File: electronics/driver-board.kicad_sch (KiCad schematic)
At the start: 62 parts, among them J10 USB_C_Receptacle_USB2.0, J2 Conn_01x02, J3 Conn_01x06, J4 Qwiic_RA, J5 Conn_02x03_Counter_Clockwise, SW1 SW_Push, SW2 SW_Push, SW3 SW_Push, SW4 SW_Push, U1 LMR16006YQ3, U2 AMS1117-3.3, U3 ESP32-C6-MINI-1/U, U5 TMC5240-TSSOP38, U7 AS5047D

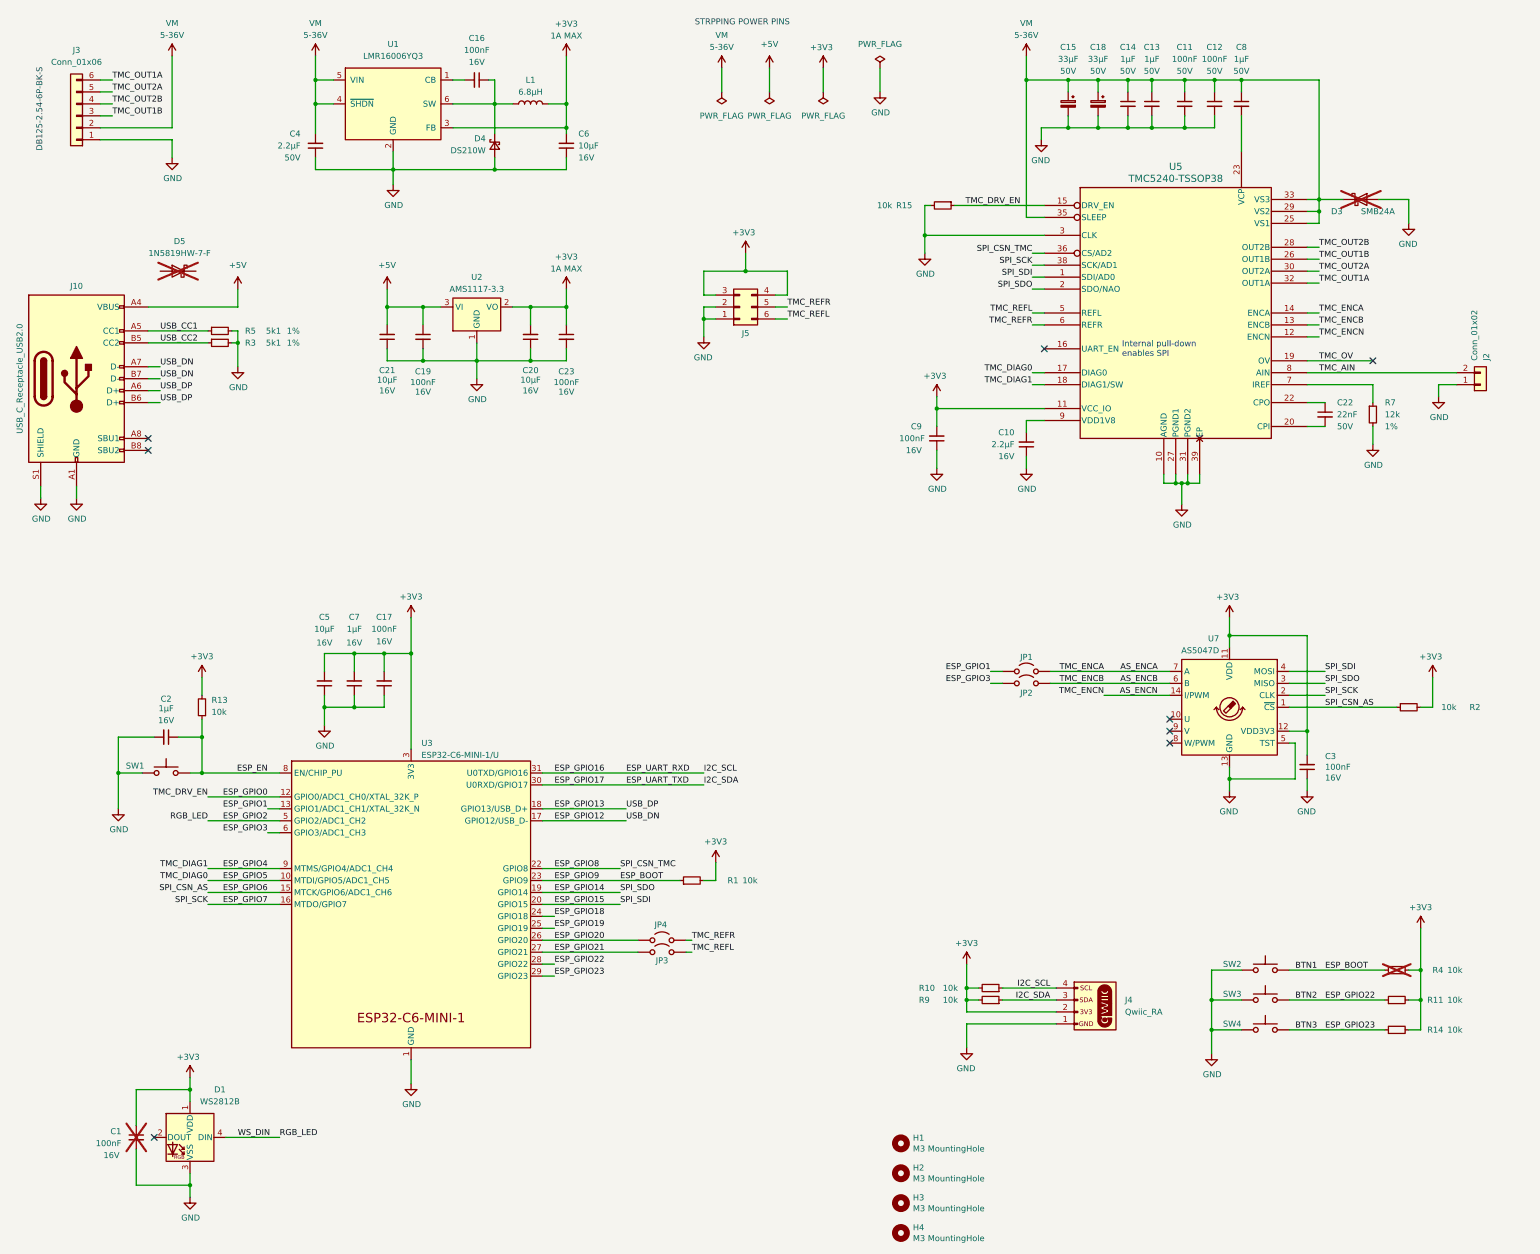
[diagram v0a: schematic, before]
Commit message: reworked layout a bit
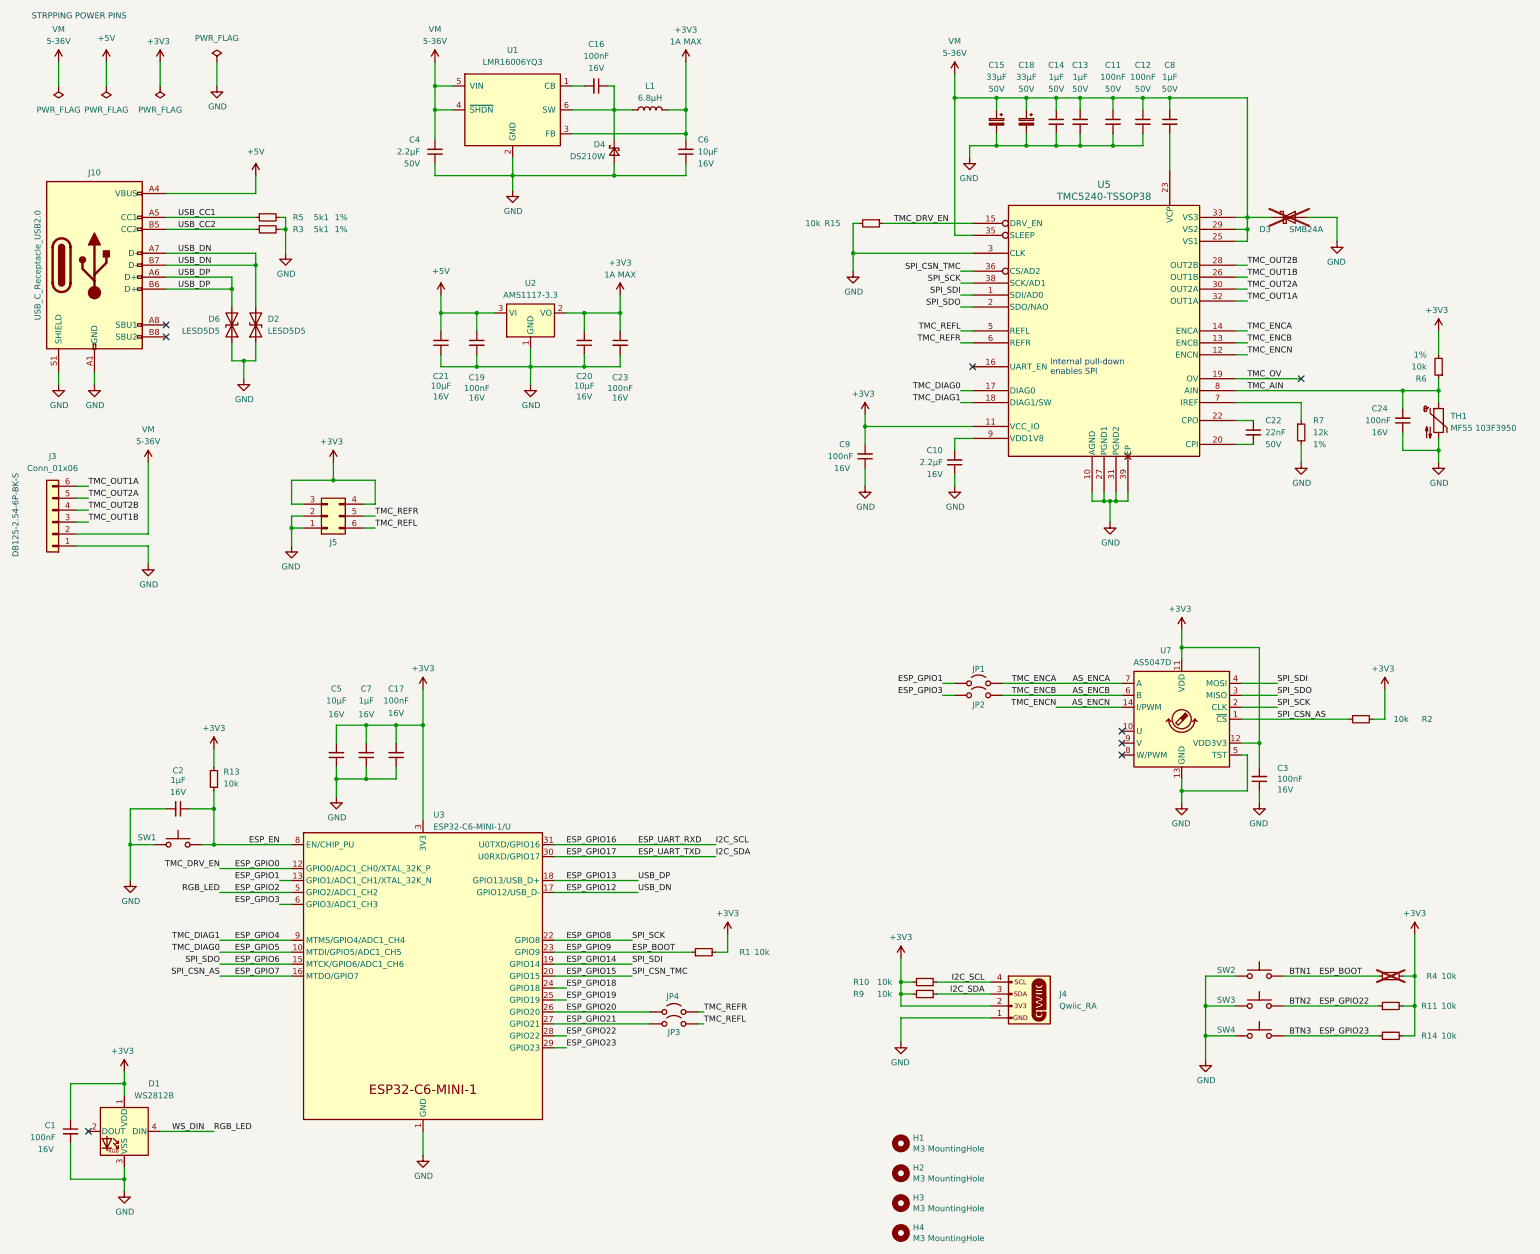
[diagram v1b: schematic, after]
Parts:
- removed D5: 1N5819HW-7-F, Diode_SMD:D_SOD-123, symbol Diode:1N5819
- removed J2: Conn_01x02, Connector_PinHeader_2.54mm:PinHeader_1x02_P2.54mm_Vertical, symbol Connector_Generic:Conn_01x02
- added C24: 100nF, Capacitor_SMD:C_0603_1608Metric, symbol Device:C_Small
- added D2, D6: LESD5D5, Diode_SMD:D_SOD-523, symbol Device:D_TVS
- added R6: 10k, Resistor_SMD:R_0402_1005Metric, symbol Device:R_Small
- added TH1: MF55 103F3950, symbol Device:Thermistor_NTC
- C1: footprint Capacitor_SMD:C_0603_1608Metric -> Capacitor_SMD:C_0402_1005Metric; now fitted; now in the parts list
- R1, R10, R11, R13, R14, R15, R2, R3, R4, R5, R9: footprint Capacitor_SMD:C_0402_1005Metric -> Resistor_SMD:R_0402_1005Metric
- R7: footprint Resistor_SMD:R_0603_1608Metric -> Resistor_SMD:R_0402_1005Metric
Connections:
- net +3V3: now also R6.2
- net ESP_GPIO12: now also D2.2 (A2)
- net ESP_GPIO13: now also D6.2 (A2)
- net ESP_GPIO14: now also U5.1 (SDI/AD0), U7.4 (MOSI); no longer U5.2 (SDO/NAO), U7.3 (MISO)
- net ESP_GPIO15: now also U5.36 (CS/AD2); no longer U5.1 (SDI/AD0), U7.4 (MOSI)
- net ESP_GPIO6: now also U5.2 (SDO/NAO), U7.3 (MISO); no longer R2.1, U7.1 (~{CS})
- net ESP_GPIO7: now also R2.1, U7.1 (~{CS}); no longer U5.38 (SCK/AD1), U7.2 (CLK)
- net ESP_GPIO8: now also U5.38 (SCK/AD1), U7.2 (CLK); no longer U5.36 (CS/AD2)
- net GND: now also C24.1, D2.1 (A1), D6.1 (A1), TH1.2
- net TMC_AIN: now also C24.2, R6.1, TH1.1
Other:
- moved on the sheet: C10, C11, C12, C13, C14, C15, C16, C17, C18, C19, C2, C20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
